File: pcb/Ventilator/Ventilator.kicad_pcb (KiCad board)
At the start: 2 copper layers, 79 parts, among them J1 Conn_02x03_Top_Bottom, J2 Screw_Terminal_01x08, J3 Screw_Terminal_01x08, J4 Screw_Terminal_01x02, K1 FINDER-40.52.7.012.0000, K2 FINDER-40.52.7.012.0000, K3 FINDER-40.52.7.012.0000, Q1 NUD3160, Q2 NUD3160, Q3 NUD3160, SW1 Reset, U1 Pico, U2 4N25, U3 4N25, U4 4N25, U5 4N25

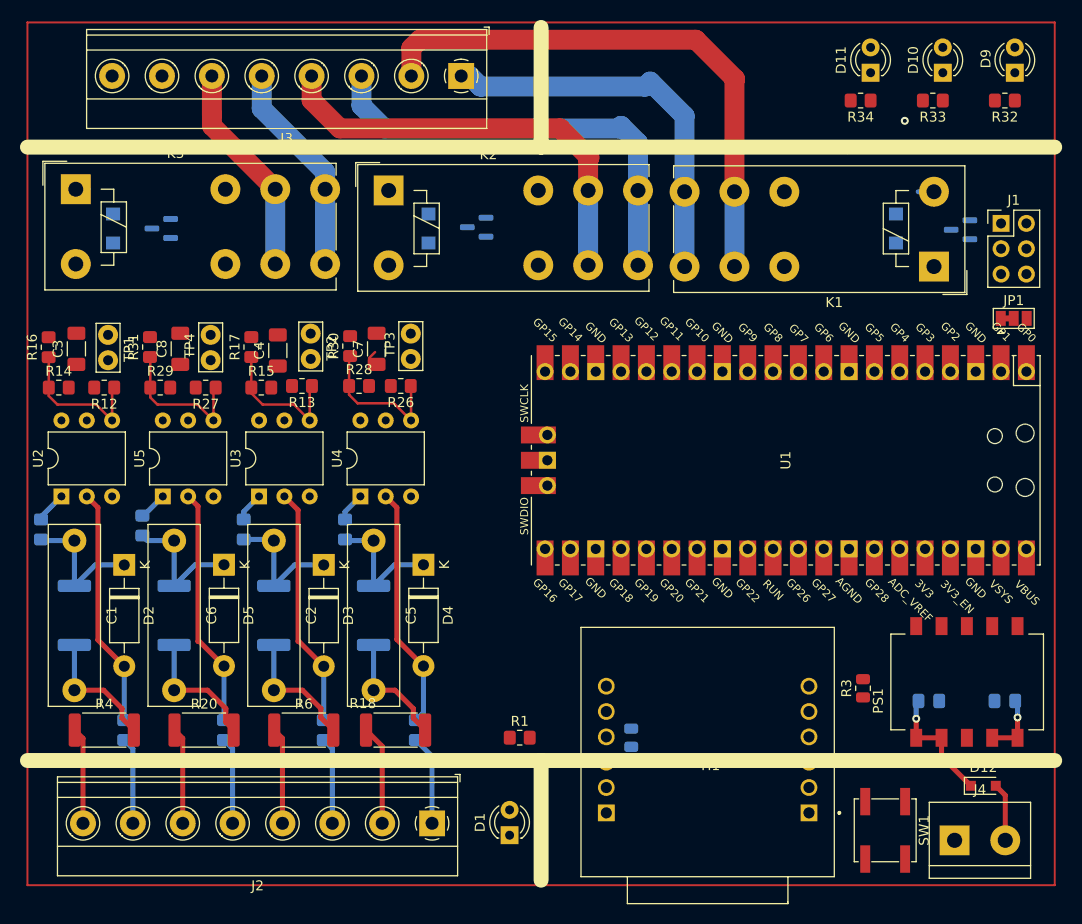
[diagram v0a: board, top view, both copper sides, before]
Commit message: - as ordered (30/12/2022)
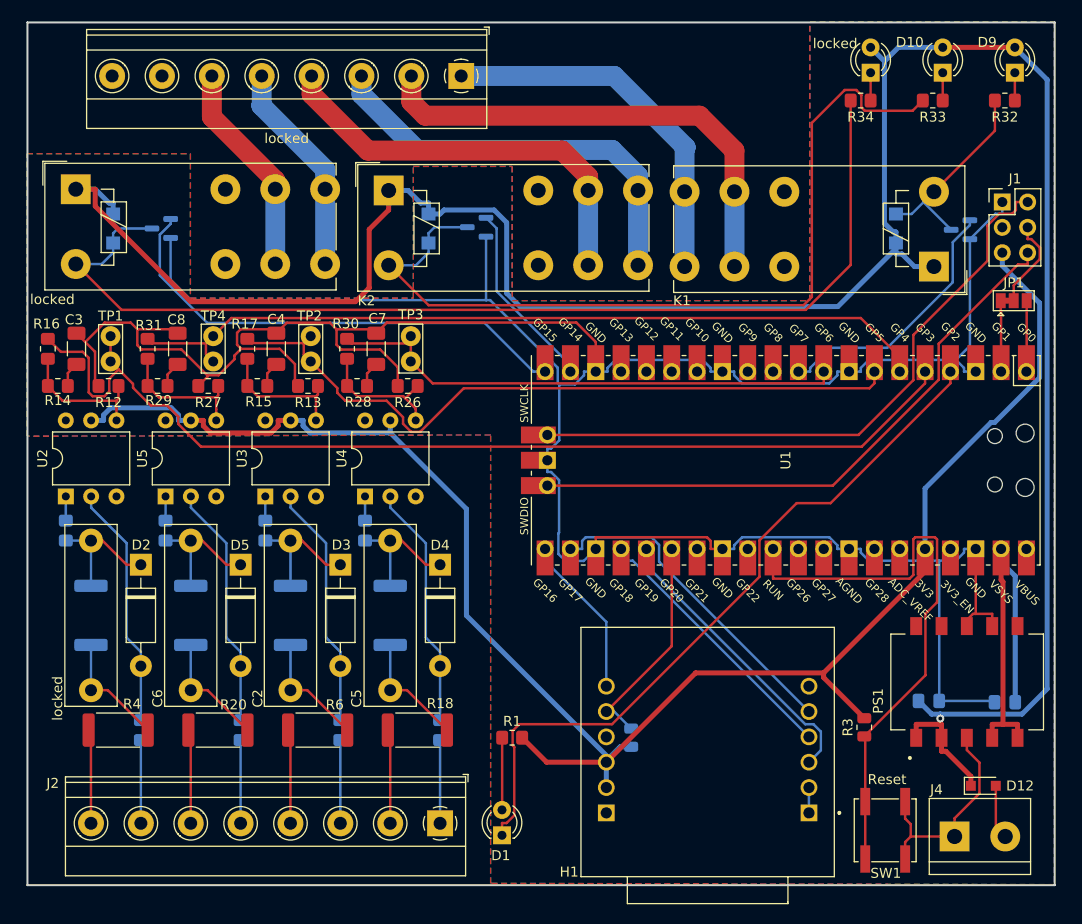
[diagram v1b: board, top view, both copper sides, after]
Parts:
- moved R3 3.92 mm to (120.9, 171.2)
- moved R10 2.49 mm to (40.8, 151.4)
- moved R19 2.43 mm to (78.4, 171.4)
- moved R25 2.38 mm to (50.8, 151.4)
- moved R18 2.18 mm to (76.1, 171.4)
- moved R11 2.17 mm to (60.8, 151.4)
- moved J1 2.15 mm to (134.7, 118.5)
- moved R24 2.01 mm to (70.8, 151.4)
- moved JP1 1.78 mm to (135.9, 128.4)
- moved D3 1.67 mm to (68.4, 154.9)
- moved D2 1.67 mm to (48.4, 154.9)
- moved C5 1.67 mm to (73.4, 152.4)
- moved D4 1.67 mm to (78.4, 154.9)
- moved R22 1.67 mm to (73.4, 159.9)
- moved R7 1.67 mm to (68.4, 171.4)
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- renumbered K3 to locked, J3 to locked, D11 to locked, C1 to locked
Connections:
- net Net-(J3-Pad1) renamed /Output/220_1
- net Net-(K1-Pad11) renamed /Output/220_2
- net Net-(K2-Pad11) renamed /Output/220_4
- net Net-(K2-Pad14) renamed /Output/220_3
- net Net-(K3-Pad11) renamed /Output/220_6
- net Net-(K3-Pad14) renamed /Output/220_5
- U1 pad 11: /CPU/OUT2 -> unconnected-(U1-Pad11)
- U1 pad 19: unconnected-(U1-Pad19) -> /CPU/OUT2
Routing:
- net GND: track 0.00 -> 335.8 mm
- net +12V: track 13.9 -> 247.5 mm
- net +3.3V: track 0.00 -> 177.0 mm
- net Net-(D8-Pad2): track 0.05 -> 108.2 mm
- net /CPU/IN1: track 0.22 -> 105.6 mm
- net Net-(D7-Pad2): track 0.70 -> 87.0 mm, vias 1 -> 0
- net /CPU/IN2: track 0.18 -> 81.9 mm
- net Net-(D1-Pad1): track 0.00 -> 73.0 mm
- net /CPU/IN3: track 0.27 -> 72.2 mm
- net /CPU/SWCLK: track 0.00 -> 63.0 mm
- net /CPU/SWD: track 0.00 -> 60.6 mm
- net Net-(R3-Pad1): track 0.00 -> 58.4 mm
- net /CPU/IN4: track 0.00 -> 52.6 mm
- net /CPU/OUT3: track 0.00 -> 48.7 mm
- net /CPU/SCNN: track 0.00 -> 33.1 mm
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- added copper zone on B.Cu, net GND
- added copper zone on F.Cu, net GND
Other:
- board outline added: 103 x 86.5 mm
